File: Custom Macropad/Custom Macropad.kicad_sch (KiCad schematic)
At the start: 49 parts, among them SW1 SW_Push, SW10 SW_Push, SW11 SW_Push, SW12 SW_Push, SW13 SW_Push, SW14 SW_Push, SW15 SW_Push, SW16 SW_Push, SW2 SW_Push, SW3 SW_Push, SW4 RotaryEncoder_Switch, SW5 SW_Push, SW6 SW_Push, SW7 SW_Push, SW8 SW_Push, SW9 SW_Push, U1 MOUDLE-SEEEDUINO-XIAO

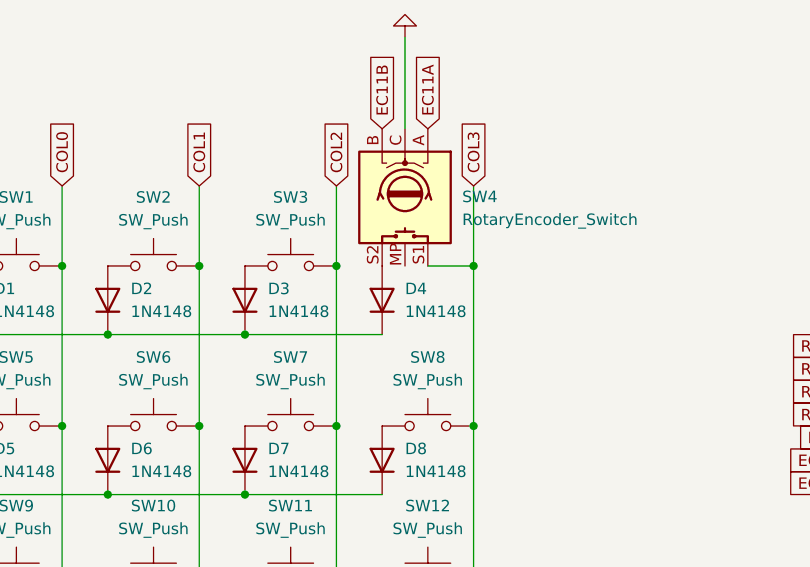
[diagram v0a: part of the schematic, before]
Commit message: Finished routing v1
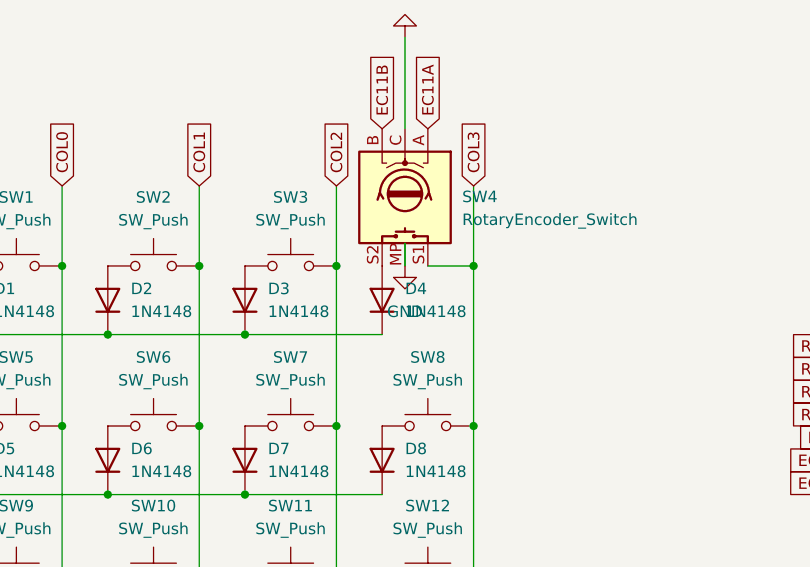
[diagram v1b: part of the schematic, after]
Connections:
- net GND: now also SW4.MP (Shield)
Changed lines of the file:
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@@
 	(wire
 		(pts
+			(xy 87.63 46.99) (xy 87.63 49.53)
+		)
+		(stroke
+			(width 0)
+			(type default)
+		)
+	)
+	(wire
+		(pts
 			(xy 78.74 113.03) (xy 57.15 113.03)
 		)
@@
 					(unit 1)
 				)
+			)
+		)
+	)
+	(symbol
+		(lib_id "power:GND")
+		(at 87.63 49.53 0)
+		(unit 1)
+		(exclude_from_sim no)
+		(in_bom yes)
+		(on_board yes)
+		(dnp no)
+		(fields_autoplaced yes)
+		(property "Reference" "#PWR07"
+			(at 87.63 55.88 0)
+			(effects
+				(font
+					(size 1.27 1.27)
+				)
+				(hide yes)
+			)
+		)
+		(property "Value" "GND"
+			(at 87.63 54.61 0)
+			(effects
+				(font
+					(size 1.27 1.27)
+				)
+			)
+		)
+		(property "Footprint" ""
+			(at 87.63 49.53 0)
+			(effects
+				(font
+					(size 1.27 1.27)
+				)
+				(hide yes)
+			)
+		)
+		(property "Datasheet" ""
+			(at 87.63 49.53 0)
+			(effects
+				(font
+					(size 1.27 1.27)
+				)
+				(hide yes)
+			)
+		)
+		(property "Description" "Power symbol creates a global label with name \"GND\" , ground"
+			(at 87.63 49.53 0)
+			(effects
+				(font
+					(size 1.27 1.27)
+				)
+				(hide yes)
+			)
+		)
+		(pin "1"
+		)
+		(instances
+			(project ""
+				(path "/cac26fb3-9366-413f-8bbf-885ac1b417bf"
+					(reference "#PWR07")
+					(unit 1)
+				)
